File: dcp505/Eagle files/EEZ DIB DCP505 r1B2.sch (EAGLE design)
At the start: 323 parts, among them IC1 LP2951, IC10 OPA4197IDR, IC11 MC33272ADR2G, IC12 MC33274ADR2G, IC13 74HC4066PW, IC14 74AUP1G74DC.125, IC15 MCP23S17-E/SS, IC16 REF5025AIDG4, IC17 DAC8552IDGKTG4, IC18 SN74LVC1G3157, IC19 ADS1120IPWR, IC2 SI8641AB-B-IS1, IC20 LM339D, IC21 LM211PWR, IC3 SN74LVC1G139DCUR, IC4 MC79L05, IC5 SI8641AB-B-IS1, IC6 AT24C02D-SSHM-T, IC7 TC77-5.0MCTTR, IC8 TL072D, IC9 MC33274ADR2G, J1 FCR7350R, J2 FCR7350B, K1 G6K-2F-5DC, Q1 IRFP250N, Q10 MMBT5551, Q11 PSMN0R9-25YLC, Q12 PSMN0R9-25YLC, Q13 PSMN0R9-25YLC, Q14 2N7002, Q15 2N7002, Q16 MMBT5401, Q17 MMBT5401, Q18 2N7002, Q19 IRLML2246TRPBF, Q2 BCP56-16.115, Q20 BTA26-600, Q21 2N7002, Q22 MMBT5551, Q23 2N7002, Q24 2N7002, Q25 MMBT5551, Q26 MMBT5551, Q27 MMBT5401, Q28 MMBT5551, Q29 MMBT5551, Q3 BC856C, Q30 BSS84P, Q31 2N7002, Q4 BCP56-16.115, Q5 STF10P6F6 or IRF9Z24 or FQPF2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, Q6 BCP56-16.115, Q7 MMBT5401, Q8 MMBT5401, Q9 MMBT5551, X1 ZL263-26DG, X2 22-05-7085, X3 39-30-3035, X4 1844249, X5 ZL263-20DG

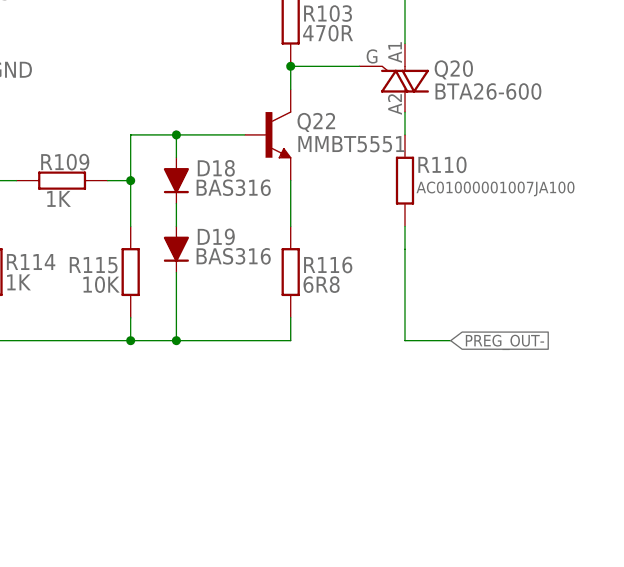
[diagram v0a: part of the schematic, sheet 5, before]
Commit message: small PCB optimizations
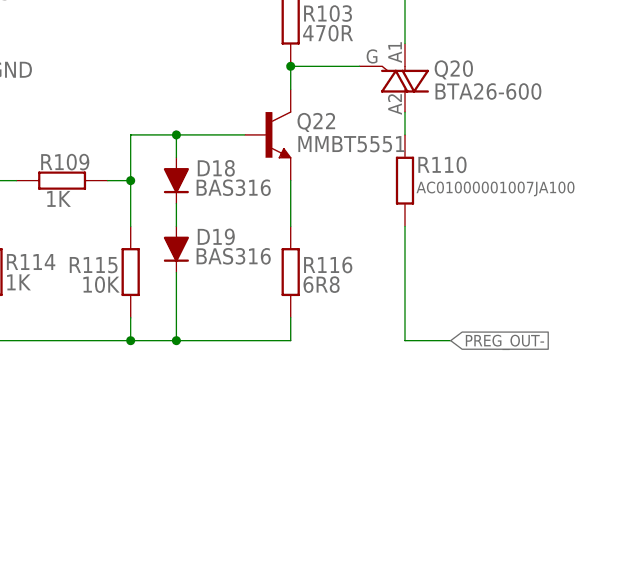
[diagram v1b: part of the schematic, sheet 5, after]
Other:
- note added: "-"
- note added: "PCB inductor ~1.1 uH !"
- note removed: "Extra Cout"
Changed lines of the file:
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@@
 <setting verticaltext="up"/>
 </settings>
-<grid distance="0.1" unitdist="inch" unit="inch" style="lines" multiple="1" display="no" altdistance="0.01" altunitdist="inch" altunit="inch"/>
+<grid distance="25" unitdist="mil" unit="mil" style="lines" multiple="4" display="no" altdistance="0.01" altunitdist="inch" altunit="inch"/>
 <layers>
 <layer number="1" name="Top" color="4" fill="1" visible="no" active="no"/>
@@
 <text x="46.99" y="115.57" size="1.4224" layer="104">Require SPI_MODE0</text>
 <text x="252.73" y="131.445" size="1.6764" layer="103" align="bottom-center">Output</text>
-<text x="252.73" y="128.905" size="1.6764" layer="103" align="bottom-center">Output</text>
+<text x="252.73" y="128.905" size="1.6764" layer="103" align="bottom-center">Input</text>
 <text x="213.36" y="144.145" size="1.6764" layer="103" align="bottom-center">6</text>
 <text x="213.36" y="136.525" size="1.6764" layer="103" align="bottom-center">9</text>
@@
 <text x="218.44" y="123.825" size="1.6764" layer="103">Current range 50 mA</text>
 <text x="213.36" y="133.985" size="1.6764" layer="103" align="bottom-center">10</text>
-<text x="252.73" y="126.365" size="1.6764" layer="103" align="bottom-center">Output</text>
+<text x="252.73" y="126.365" size="1.6764" layer="103" align="bottom-center">Input</text>
 <text x="188.595" y="107.315" size="1.27" layer="100">+2.5 V</text>
 <text x="213.36" y="121.285" size="1.6764" layer="103" align="bottom-center">15</text>
-<text x="218.44" y="121.285" size="1.6764" layer="103">Extra Cout</text>
-<text x="252.73" y="121.285" size="1.6764" layer="103" align="bottom-center">Output</text>
+<text x="218.44" y="121.285" size="1.6764" layer="103">-</text>
+<text x="252.73" y="121.285" size="1.6764" layer="103" align="bottom-center">-</text>
 <text x="218.44" y="141.605" size="1.6764" layer="103">OE coupled LED</text>
 <text x="213.36" y="131.445" size="1.6764" layer="103" align="bottom-center">11</text>
@@
 <text x="213.36" y="126.365" size="1.6764" layer="103" align="bottom-center">13</text>
 <text x="213.36" y="123.825" size="1.6764" layer="103" align="bottom-center">14</text>
-<text x="252.73" y="123.825" size="1.6764" layer="103" align="bottom-center">Output</text>
+<text x="252.73" y="123.825" size="1.6764" layer="103" align="bottom-center">Input</text>
 <text x="252.73" y="136.525" size="1.6764" layer="103" align="bottom-center">Output</text>
 <text x="119.38" y="12.065" size="1.6764" layer="103">AIN0</text>
@@
 <rectangle x1="141.605" y1="119.38" x2="148.59" y2="126.365" layer="97"/>
 <wire x1="119.38" y1="83.82" x2="119.38" y2="172.72" width="0.1524" layer="97" style="shortdash"/>
+<wire x1="243.84" y1="121.92" x2="240.665" y2="121.92" width="0.1524" layer="100"/>
+<polygon width="0.1524" layer="100">
+<vertex x="240.665" y="121.92"/>
+<vertex x="241.935" y="122.2375"/>
+<vertex x="241.935" y="121.6025"/>
+</polygon>
+<text x="244.475" y="120.3325" size="1.27" layer="100">PCB inductor
+~1.1 uH !</text>
+<wire x1="237.49" y1="127" x2="240.03" y2="127" width="0.1524" layer="100"/>
+<wire x1="240.03" y1="127" x2="240.03" y2="115.57" width="0.1524" layer="100"/>
+<wire x1="240.03" y1="115.57" x2="237.49" y2="115.57" width="0.1524" layer="100"/>
+<wire x1="237.49" y1="115.57" x2="237.49" y2="127" width="0.1524" layer="100"/>
 </plain>
 <instances>
@@
 <label x="243.84" y="114.3" size="1.27" layer="102" xref="yes"/>
 <pinref part="R110" gate="G$1" pin="1"/>
-<wire x1="238.76" y1="127" x2="238.76" y2="124.46" width="0.4064" layer="91"/>
-<wire x1="238.76" y1="114.3" x2="238.76" y2="124.46" width="0.1524" layer="91"/>
+<wire x1="238.76" y1="127" x2="238.76" y2="114.3" width="0.4064" layer="91"/>
 </segment>
 </net>
@@
 </schematic>
 </drawing>
+<compatibility>
+<note version="6.3" minversion="6.2.2" severity="warning">
+Since Version 6.2.2 text objects can contain more than one line,
+which will not be processed correctly with this version.
+</note>
+</compatibility>
 </eagle>
